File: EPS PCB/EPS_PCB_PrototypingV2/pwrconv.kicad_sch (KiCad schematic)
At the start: 30 parts, among them J3 Conn_01x02_Pin, J4 Conn_01x02_Pin, J5 Conn_01x02_Pin, U1 TPS5430DDA, U2 TPS5430DDA, U3 TPS5430DDA

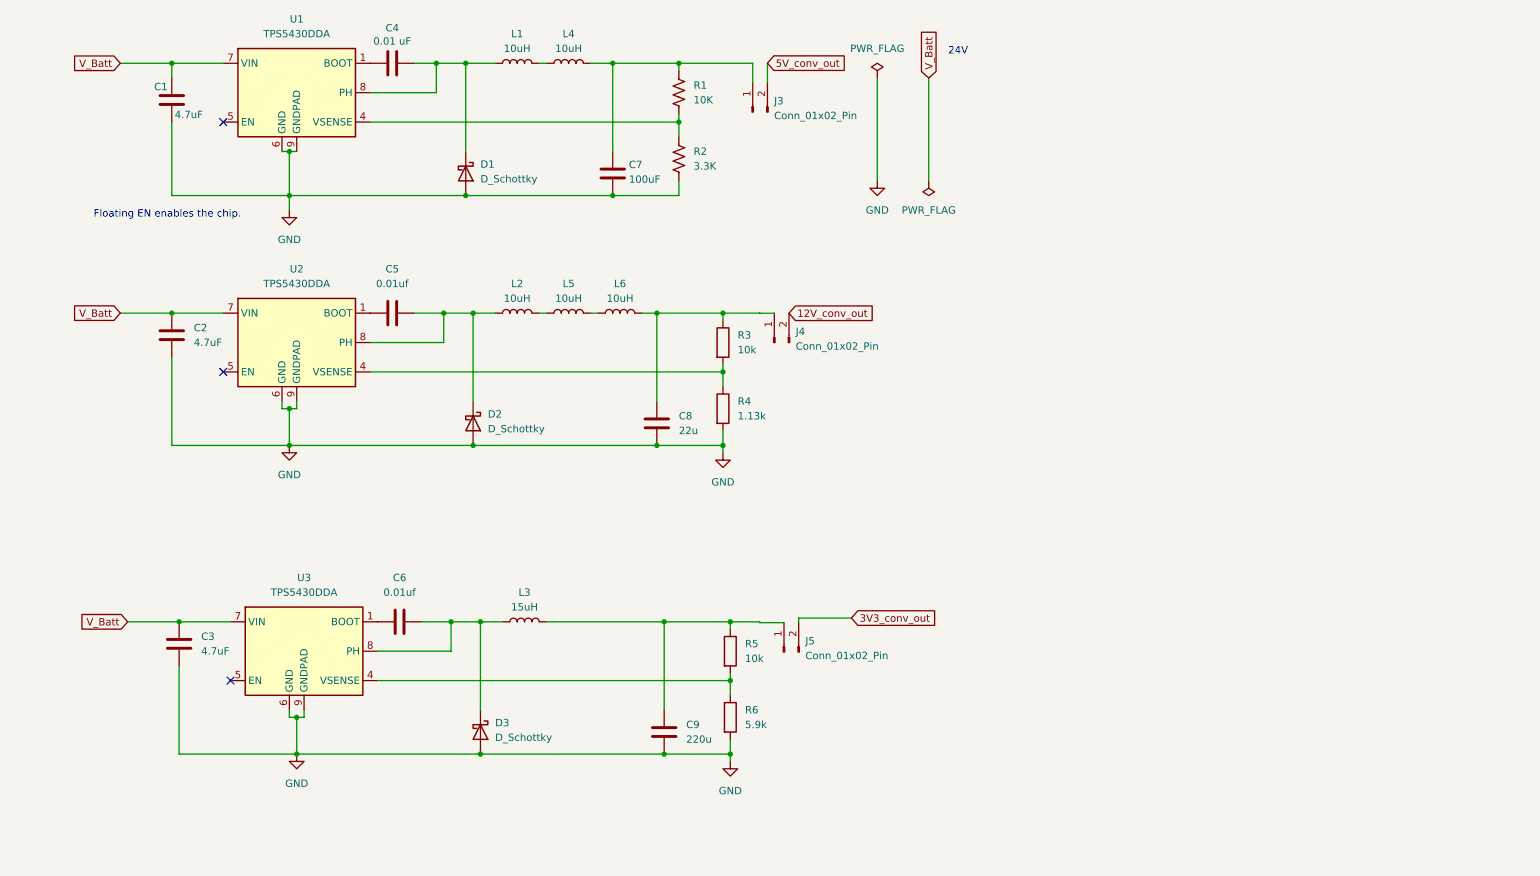
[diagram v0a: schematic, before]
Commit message: PC104 Template Updates
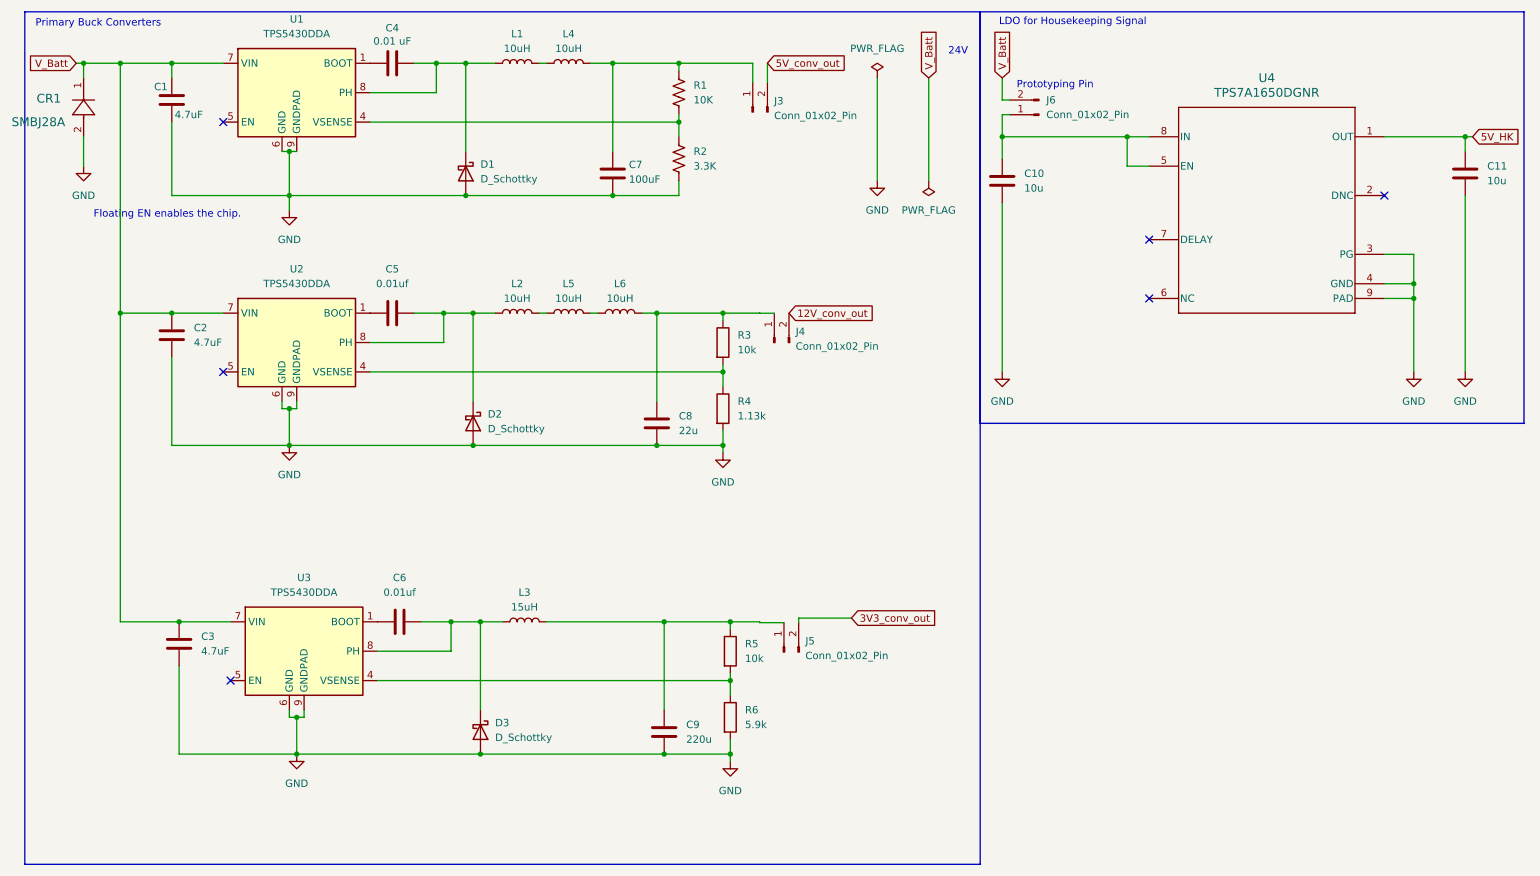
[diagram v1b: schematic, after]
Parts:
- added C10, C11: 10u, Capacitor_SMD:C_0603_1608Metric, symbol Device:C
- added CR1: SMBJ28A, Footprints:DIODE_DO214AA, symbol SMBJ28A:SMBJ28A
- added J6: Conn_01x02_Pin, Connector_PinSocket_2.54mm:PinSocket_1x02_P2.54mm_Vertical, symbol Connector:Conn_01x02_Pin
- added U4: TPS7A1650DGNR, Footprints:DGN0008C_N, symbol TPS6A1650DGNR:TPS7A1650DGNR
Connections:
- net GND: now also C10.1, C11.1, CR1.2, U4.3 (PG), U4.4 (GND), U4.9 (PAD)
- net V_Batt: now also CR1.1, J6.2 (Pin_2)
- new net: C10.2, J6.1 (Pin_1), U4.5 (EN), U4.8 (IN)
- new net 5V_HK: C11.2, U4.1 (OUT)
- no-connect marks 3 -> 6
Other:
- note added: "LDO for Housekeeping Signal"
- note added: "Primary Buck Converters"
- note added: "Prototyping Pin"
